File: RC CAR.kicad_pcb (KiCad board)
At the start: 2 copper layers, 70 x 60 mm, 13 parts, among them J1 RW, J2 LW, J4 US, J5 RGB, J6 J2, J7 J2, U1 L293D, U2 ESP32-DEVKIT-V1, U3 L7805

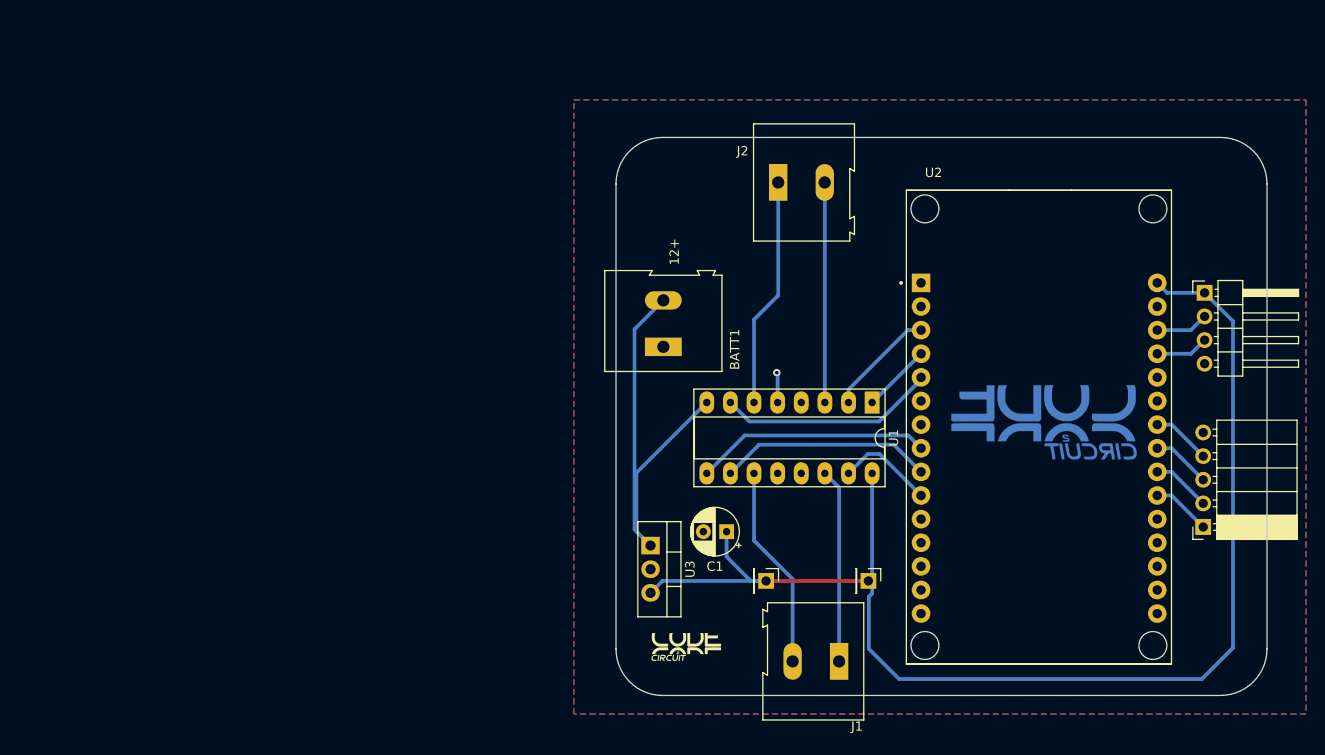
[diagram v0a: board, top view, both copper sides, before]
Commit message: Raspberry Pico Dev-Board Copy
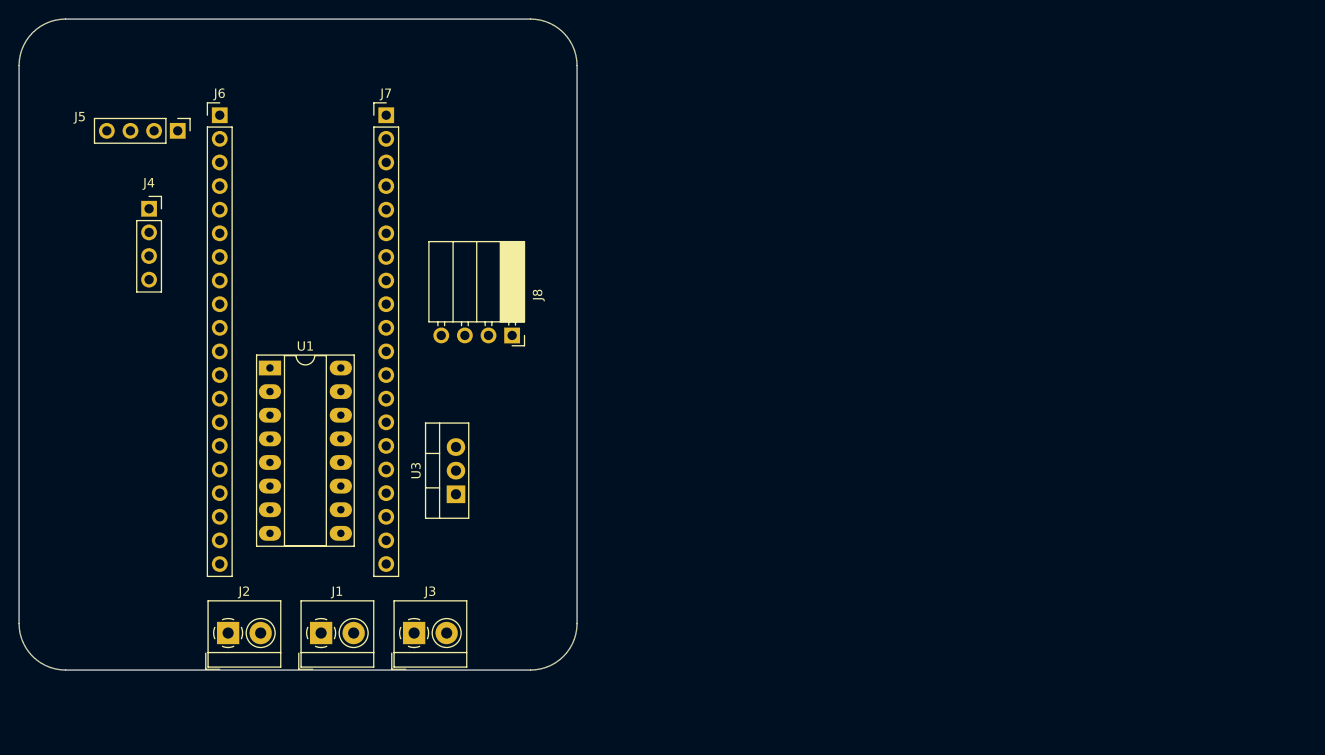
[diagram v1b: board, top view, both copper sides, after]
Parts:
- removed BATT1: J3, TerminalBlock:TerminalBlock_Altech_AK300-2_P5.00mm
- removed C1: CPS, Capacitor_THT:CP_Radial_D5.0mm_P2.50mm
- removed the G*** at (107.2, 125.0)
- removed the G*** at (145.8, 100.8)
- removed U2: ESP32-DEVKIT-V1, MODULE_ESP32_DEVKIT_V1:MODULE_ESP32_DEVKIT_V1
- added G***: LOGO, LOGO, B.Cu at (64.1, 81.9)
- added J3: BATT, TerminalBlock_4Ucon:TerminalBlock_4Ucon_1x02_P3.50mm_Horizontal, F.Cu at (78.0, 123.5)
- added J8: HC-06, Connector_PinSocket_2.54mm:PinSocket_1x04_P2.54mm_Horizontal, F.Cu at (88.5, 91.5)
- J1, J2: footprint TerminalBlock:TerminalBlock_Altech_AK300-2_P5.00mm -> TerminalBlock_4Ucon:TerminalBlock_4Ucon_1x02_P3.50mm_Horizontal
- J4: value US -> RGB; footprint Connector_PinHeader_2.54mm:PinHeader_1x04_P2.54mm_Horizontal -> Connector_PinSocket_2.54mm:PinSocket_1x04_P2.54mm_Vertical
- J5: value RGB -> US; footprint Connector_PinSocket_2.54mm:PinSocket_1x05_P2.54mm_Horizontal -> Connector_PinHeader_2.54mm:PinHeader_1x04_P2.54mm_Vertical
- J6, J7: value J2 -> Conn_01x20; footprint Connector_PinHeader_2.54mm:PinHeader_1x01_P2.54mm_Vertical -> Connector_PinHeader_2.54mm:PinHeader_1x20_P2.54mm_Vertical
- moved J5 118.2 mm to (52.6, 69.5), turned to -90 degrees
- moved J4 113.9 mm to (49.5, 77.9)
- moved J6 77.2 mm to (57.1, 67.8), turned to 0 degrees
- moved J2 76.5 mm to (58.0, 123.5)
- moved J7 72.1 mm to (75.0, 67.8), turned to 0 degrees
- moved U1 64.9 mm to (62.5, 95.0), turned to 0 degrees
- moved J1 55.8 mm to (68.0, 123.5), turned to 0 degrees
- moved U3 21.6 mm to (82.5, 108.6), turned to 90 degrees
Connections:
- J1 pad 1: RW1 -> /RW1
- J1 pad 2: RW2 -> /RW2
- J2 pad 1: LW1 -> /LW1
- J2 pad 2: LW2 -> /LW2
- J4 pad 1: +5V -> GND
- J4 pad 2: TRIG -> /R
- J4 pad 3: ECHO -> /G
- J4 pad 4: GND -> /B
- J5 pad 1: L -> GND
- J5 pad 2: B -> /Trig
- J5 pad 3: G -> /Echo
- J5 pad 4: R -> +5V
- J6 pad 1: +5V -> /Echo
- U1 pad 1: ENA -> /ENA
- U1 pad 10: IN3 -> /IN3
- U1 pad 11: RW2 -> /RW1
- U1 pad 14: RW1 -> /RW2
- U1 pad 15: IN4 -> /IN4
- U1 pad 16: +5V -> +12V
- U1 pad 2: IN1 -> /IN1
- U1 pad 3: LW2 -> /LW1
- U1 pad 6: LW1 -> /LW2
- U1 pad 7: IN2 -> /IN2
- U1 pad 8: +12V -> +5V
- U1 pad 9: ENB -> /ENB
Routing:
- net +5V: track 137.9 -> 0.00 mm
- net +12V: track 45.4 -> 0.00 mm
- net ENB: track 25.3 -> 0.00 mm
- net LW1: track 24.7 -> 0.00 mm
- net LW2: track 23.7 -> 0.00 mm
- net IN2: track 23.4 -> 0.00 mm
- net IN3: track 23.0 -> 0.00 mm
- net RW2: track 21.9 -> 0.00 mm
- net RW1: track 20.9 -> 0.00 mm
- net IN1: track 11.8 -> 0.00 mm
- net IN4: track 10.5 -> 0.00 mm
- net ENA: track 7.43 -> 0.00 mm
- net R: track 6.63 -> 0.00 mm
- net L: track 6.34 -> 0.00 mm
- net G: track 6.34 -> 0.00 mm
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- removed copper zone on B.Cu, net GND
- removed copper zone on F.Cu, net GND
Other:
- board size 70 x 60 mm -> 60 x 70 mm
- board text removed: "12+"
